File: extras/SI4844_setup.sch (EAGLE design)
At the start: 24 parts, among them M1 ARDUINO-NANO-3.0

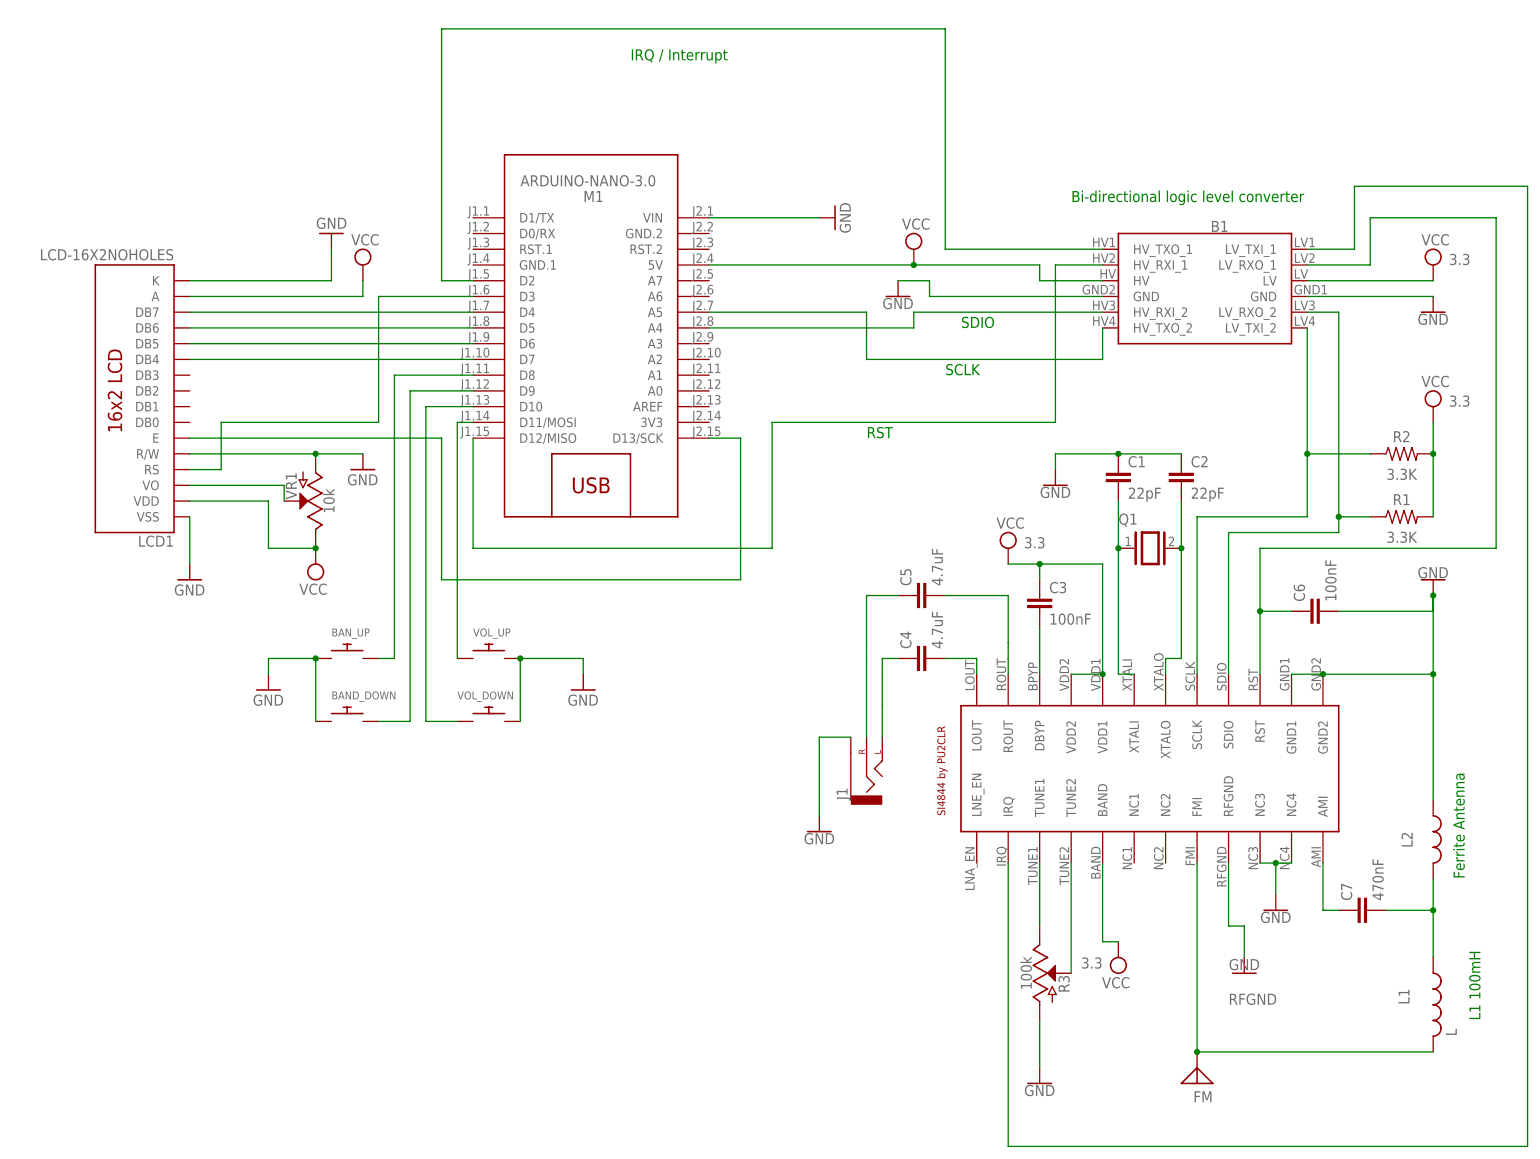
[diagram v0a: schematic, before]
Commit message: SI4844 Arduino Library
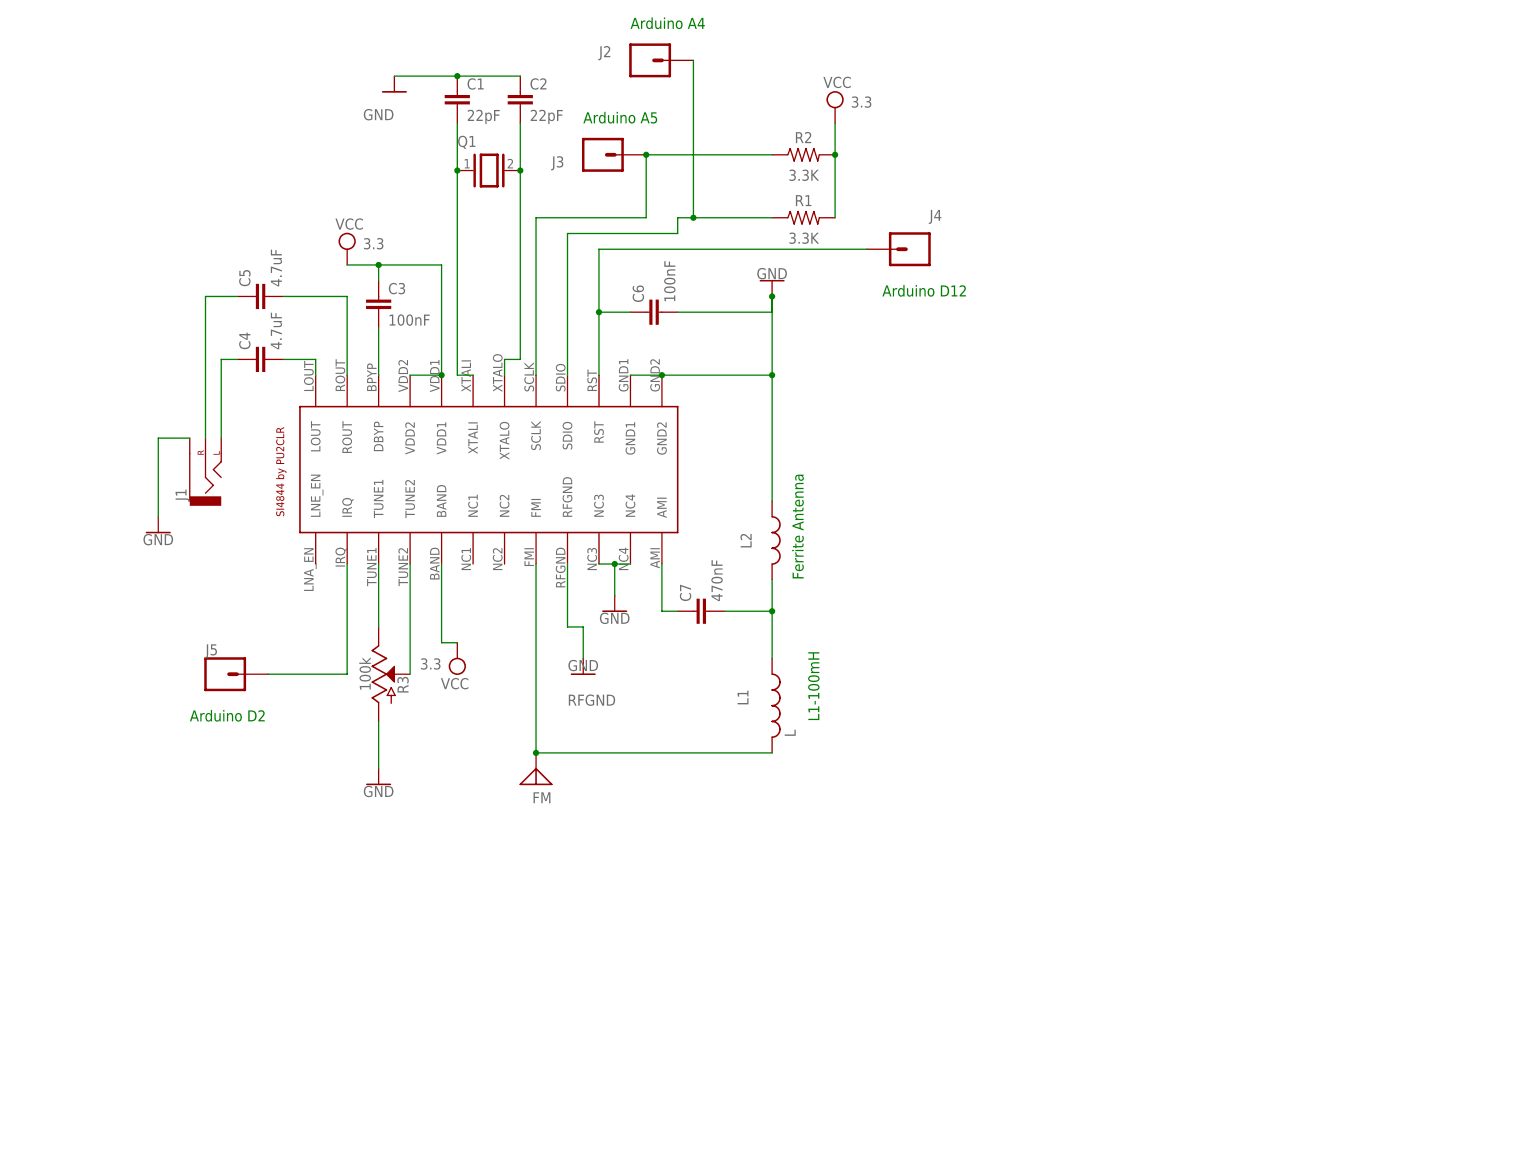
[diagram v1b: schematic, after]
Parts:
- removed B1: SPARKFUN_LOGIC_LEVEL_CONVERTERLOCK, SparkFun-Boards:SPARKFUN_LOGIC_LEVEL_CONVERTERLOCK
- removed BAND_DOWN, BAN_UP, VOL_DOWN, VOL_UP: (no value), adafruit:SWITCH_PUSHBUTTONC&K_KSS
- removed LCD1: LCD-16X2NOHOLES, SparkFun-Displays:LCD-16X2NOHOLES
- removed M1: ARDUINO-NANO-3.0, diy-modules:ARDUINO-NANO-3.0
- removed VR1: 10k, SparkFun-Resistors:POTENTIOMETER-PTH-9MM-1/20W-20%
- added J2, J3, J4, J5: (no value), SparkFun-Connectors:CONN_01
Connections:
- removed net N$10: LCD1.VO, VR1.S
- removed net N$11: LCD1.RS, M1.D3
- removed net N$19: B1.LV_TXI_2, R2.1, SI1.SCLK
- removed net N$2: LCD1.DB6, M1.D5
- removed net N$21: B1.LV_RXO_2, R1.1, SI1.SDIO
- removed net N$23: B1.HV_TXO_2, M1.A5
- removed net N$24: B1.HV_RXI_2, M1.A4
- removed net N$25: B1.LV_TXI_1, SI1.IRQ
- removed net N$26: B1.HV_TXO_1, M1.D2
- removed net N$27: B1.HV_RXI_1, M1.D12/MISO
- removed net N$3: LCD1.DB5, M1.D6
- removed net N$4: LCD1.DB4, M1.D7
- removed net N$5: BAN_UP.P$2, M1.D8
- removed net N$6: LCD1.E, M1.D13/SCK
- removed net N$7: BAND_DOWN.P$2, M1.D9
- removed net N$8: M1.D10, VOL_DOWN.P$1
- removed net N$9: M1.D11/MOSI, VOL_UP.P$1
- new net ARDUINO_A4: J2.1, R1.1, SI1.SDIO
- new net ARDUINO_A5: J3.1, R2.1, SI1.SCLK
- net GND: no longer B1.GND, B1.GND@2, BAND_DOWN.P$1, BAN_UP.P$1, LCD1.K, LCD1.R/W, LCD1.VSS, M1.VIN, VOL_DOWN.P$2, VOL_UP.P$2, VR1.A
- net N$1: now also J5.1, SI1.IRQ; no longer LCD1.DB7, M1.D4
- net N$22: now also J4.1; no longer B1.LV_RXO_1
- net VCC: no longer B1.HV, B1.LV, LCD1.A, LCD1.VDD, M1.5V, VR1.E
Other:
- note added: "Arduino A4"
- note added: "Arduino A5"
- note added: "Arduino D12"
- note added: "Arduino D2"
- note added: "L1-100mH"
- note removed: "Bi-directional logic level converter"
- note removed: "IRQ / Interrupt"
- note removed: "L1 100mH"
- note removed: "RST"
- note removed: "SCLK"
- note removed: "SDIO"
- moved on the sheet: C1, C2, C3, C4, C5, C6, C7, FM, J1, L1, L2, Q1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
